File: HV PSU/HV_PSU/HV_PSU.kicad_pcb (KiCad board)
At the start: 2 copper layers, 200 x 80 mm, 105 parts, among them J1 Screw_Terminal_01x07, J13 MountingHole_Pad, J2 AC_HV_1, J3 AC_HV_2, J4 MountingHole_Pad, J5 AC_HV_2, Q1 2N7002, Q2 IRFS4227, Q3 IRFS4227, T1 UY12, U1 L7812, U2 TPS2814D

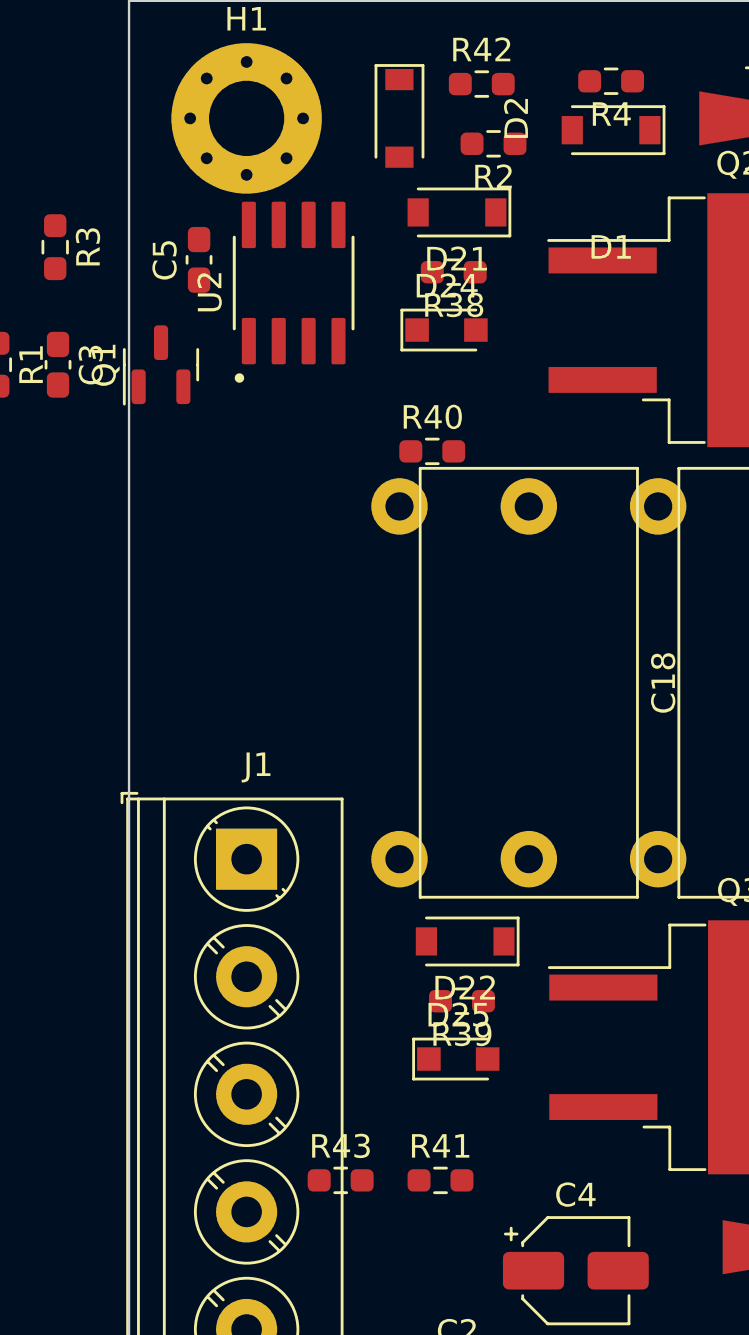
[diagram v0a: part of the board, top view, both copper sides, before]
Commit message: backup
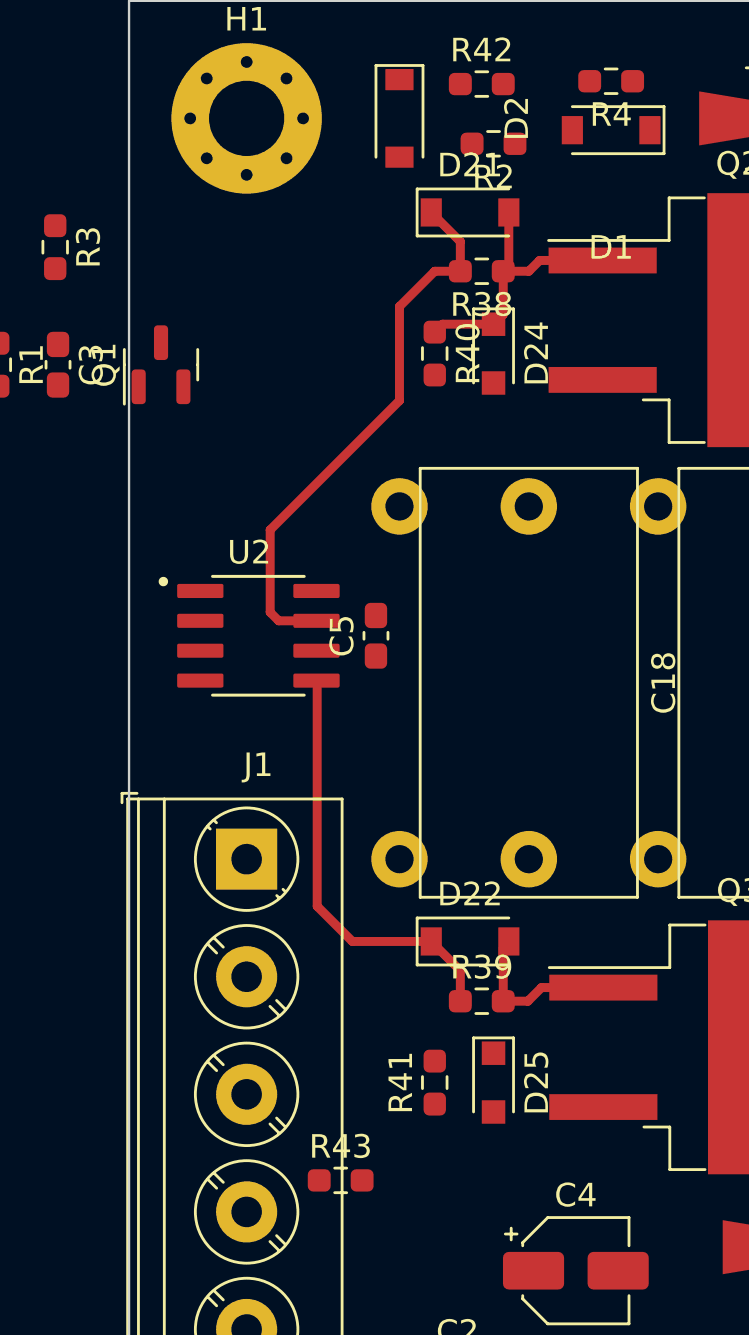
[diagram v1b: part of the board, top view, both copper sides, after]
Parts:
- moved C5 17.7 mm to (10.5, 47.0)
- moved U2 15.1 mm to (5.50, 47.0), turned to 0 degrees
- moved R41 4.17 mm to (13.0, 66.0), turned to 90 degrees
- moved R40 4.16 mm to (13.0, 35.0), turned to -90 degrees
- moved D24 2.24 mm to (15.5, 35.0), turned to -90 degrees
- moved D25 1.80 mm to (15.5, 66.0), turned to -90 degrees
- moved R38 1.19 mm to (15.0, 31.5)
- moved R39 0.84 mm to (15.0, 62.5), turned to 0 degrees
- moved D21 0.55 mm to (14.5, 29.0), turned to 0 degrees
- moved D22 0.21 mm to (14.5, 60.0), turned to 0 degrees
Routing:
- net Net-(D21-Pad1): track 0.00 -> 23.6 mm
- net Net-(D22-Pad1): track 0.00 -> 18.1 mm
- net Net-(D21-Pad2): track 0.00 -> 12.1 mm
- net Net-(D22-Pad2): track 0.00 -> 7.14 mm
